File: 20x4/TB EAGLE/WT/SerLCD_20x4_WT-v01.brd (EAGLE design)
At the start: 73.7 x 99.1 mm, 3 parts

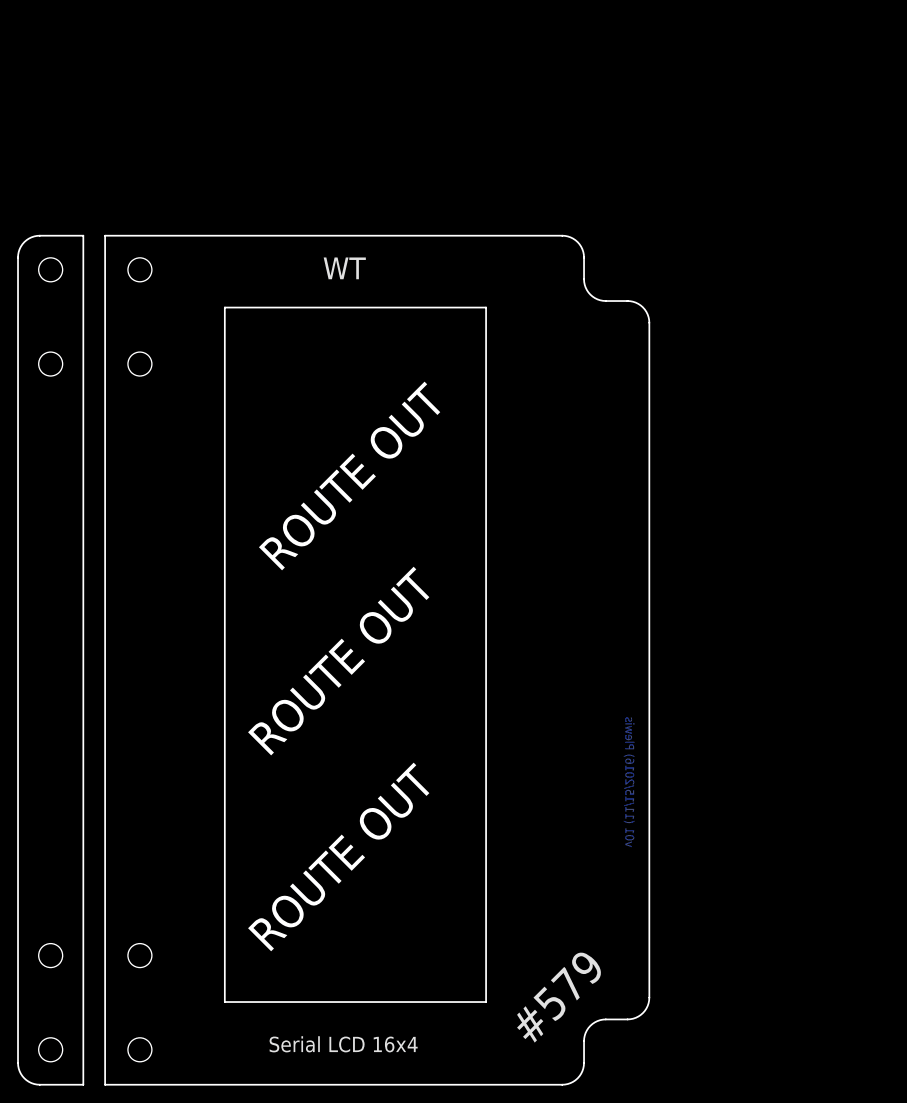
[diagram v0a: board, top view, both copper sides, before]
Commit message: finshed up 20x4, RFR
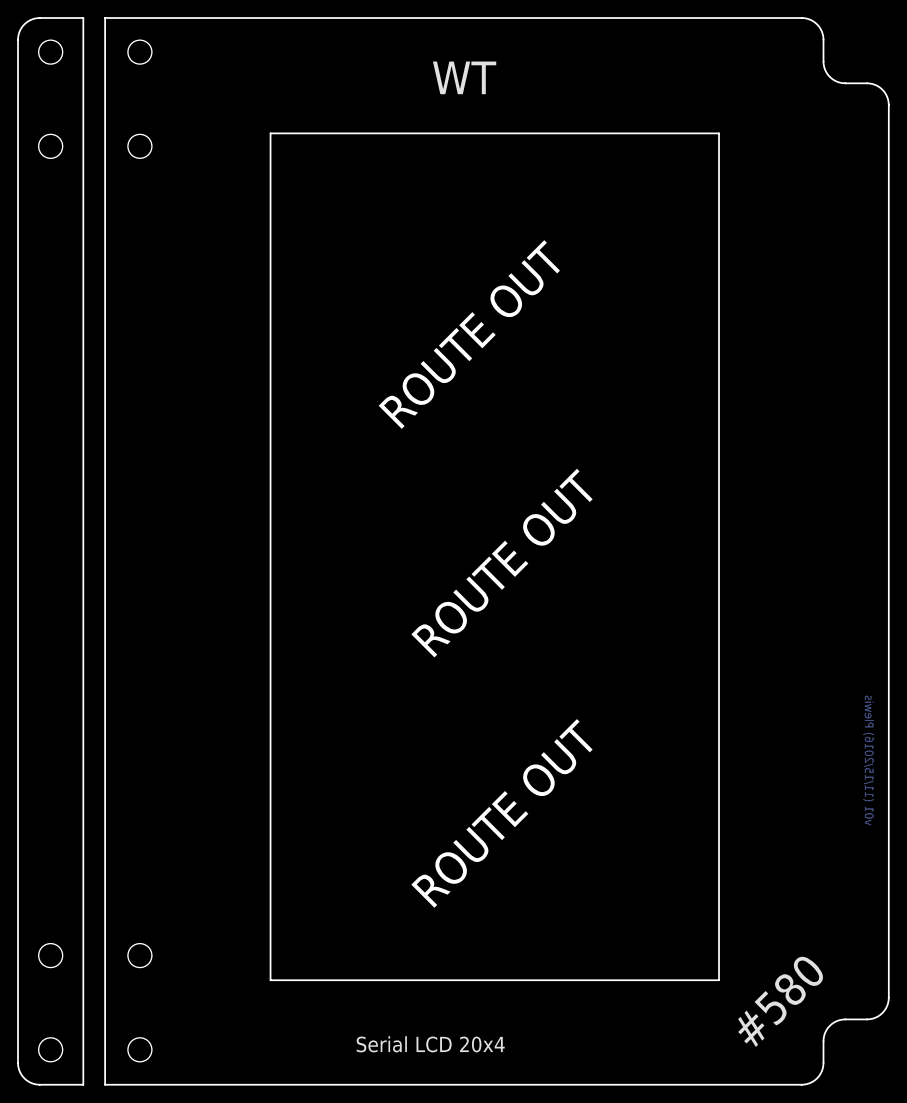
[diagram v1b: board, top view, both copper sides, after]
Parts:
- removed U$2: (no value), SerLCD_dimensions:SRE_LCD_16X2_REF_ONLY
- added U$1: (no value), SerLCD_dimensions:SER_LCD_20X4_REF_ONLY
- moved U$6 25.4 mm to (0.00, 105.4)
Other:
- board size 73.7 x 99.1 mm -> 101.6 x 124.5 mm
- board text added: "#580"
- board text added: "Serial LCD 20x4"
- board text removed: "#579"
- board text removed: "Serial LCD 16x4"
